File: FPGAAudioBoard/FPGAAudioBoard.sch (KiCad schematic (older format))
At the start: 15 parts, among them P1 QMOD-Device-x2-Type-Generic-A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, U1 CS4272

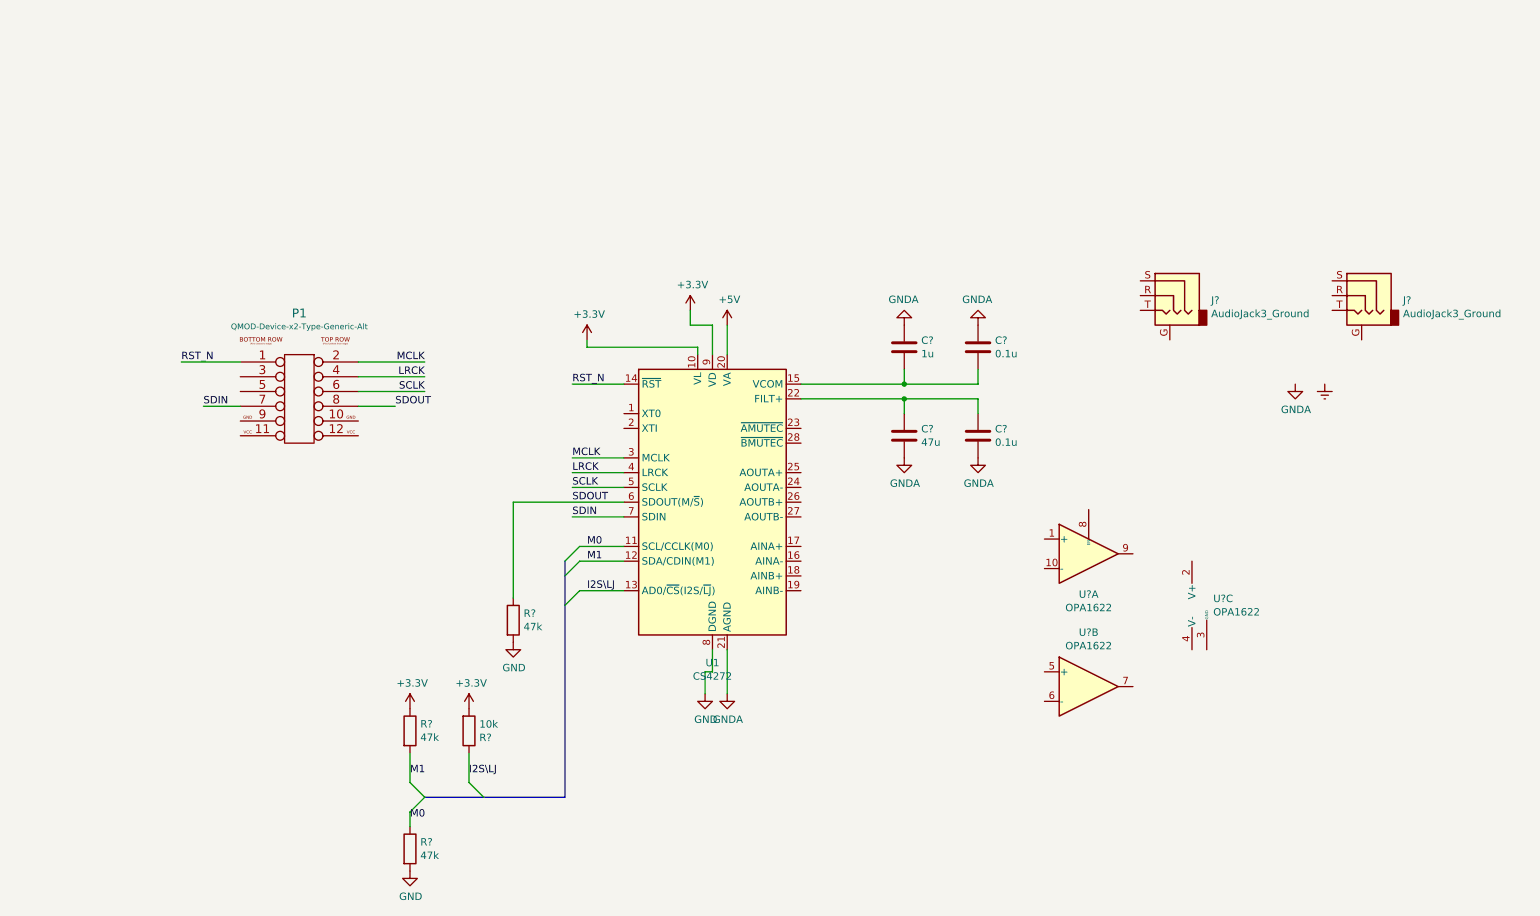
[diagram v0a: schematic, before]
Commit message: Minor changes :)
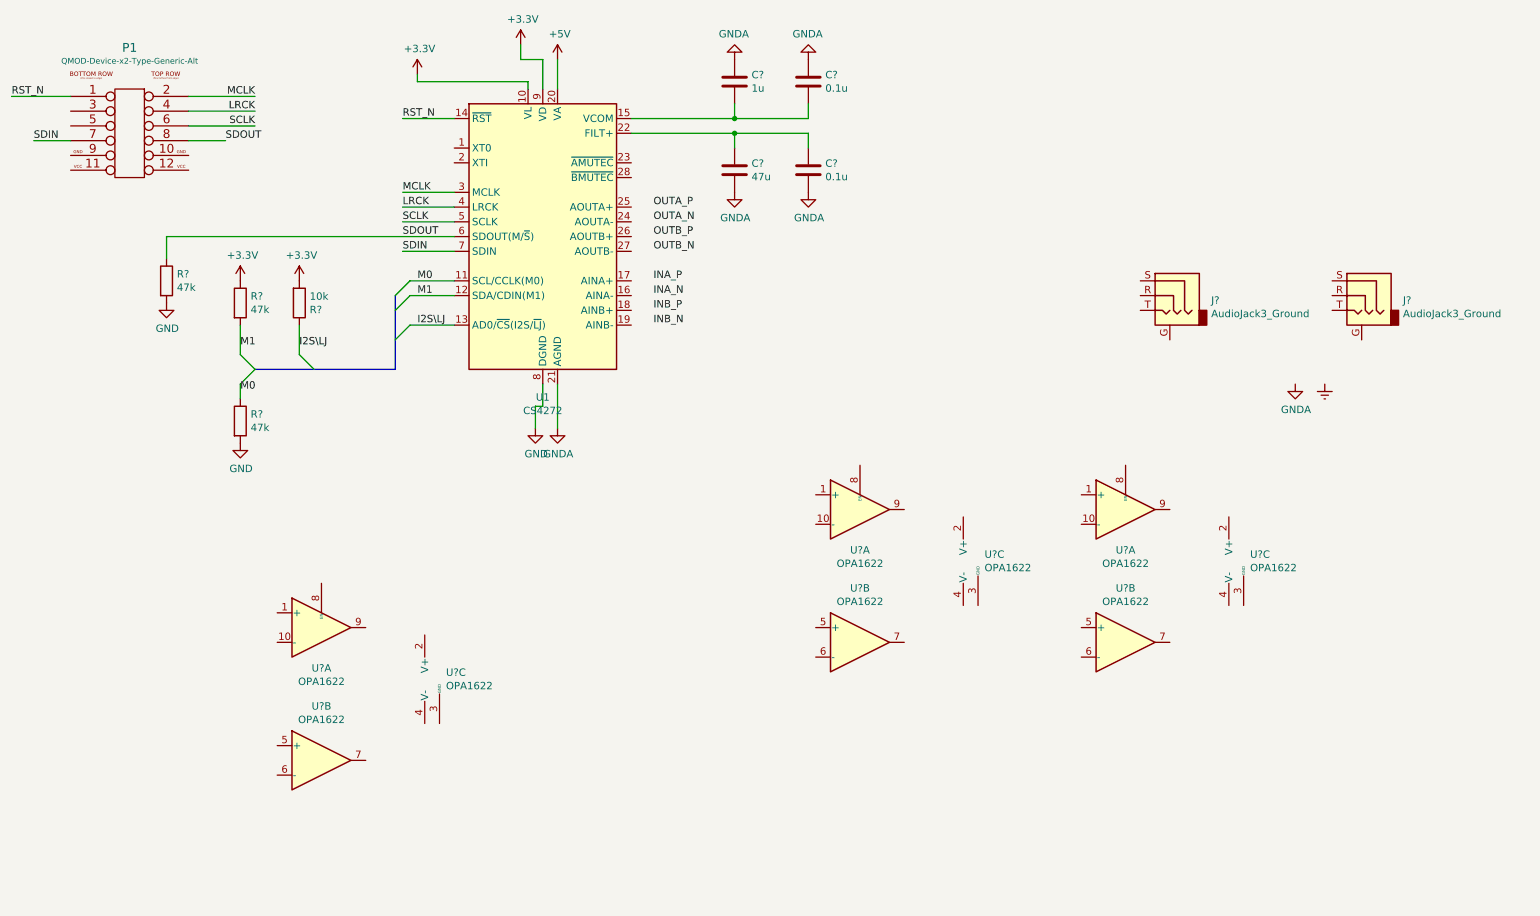
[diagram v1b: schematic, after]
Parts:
- added U? (x6): OPA1622, Package_SON:Texas_S-PVSON-N10, symbol Amplifier_Audio:OPA1622
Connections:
- new net: U?.11 (V-), U?.4 (V-) (x2)
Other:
- moved on the sheet: C?, P1, R?, U1, U?A, U?B, U?C
